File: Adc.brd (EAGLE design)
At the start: 96.8 x 28.7 mm, 98 parts, among them IC1 ADS1256IDBT, IC10 AD8605ARTZ, IC11 REF3125AIDBZT, IC12 MCP170333MB, IC2 ADUM1402ARWZ, IC3 AD8605ARTZ, IC4 AD8605ARTZ, IC5 AD8605ARTZ, IC6 AD8605ARTZ, IC7 AD8605ARTZ, IC8 AD8605ARTZ, IC9 AD8605ARTZ, Q1 7.68MHz

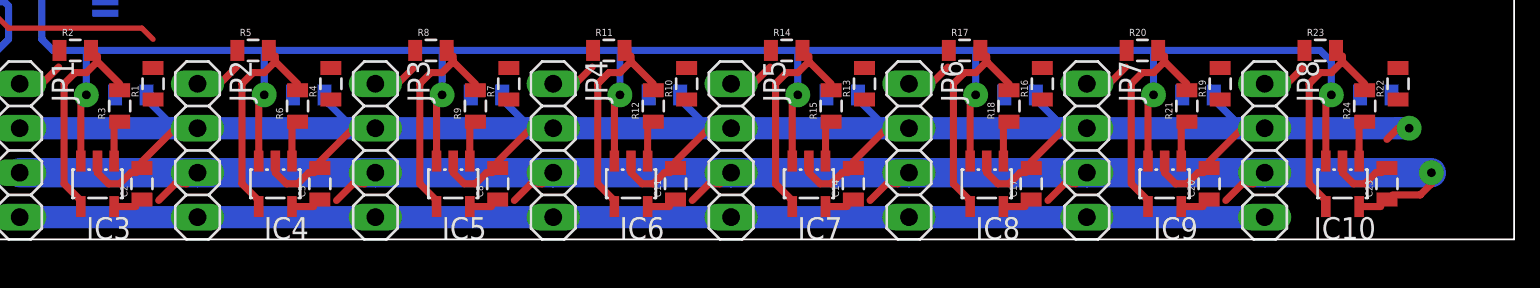
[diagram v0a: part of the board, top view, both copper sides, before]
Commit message: .
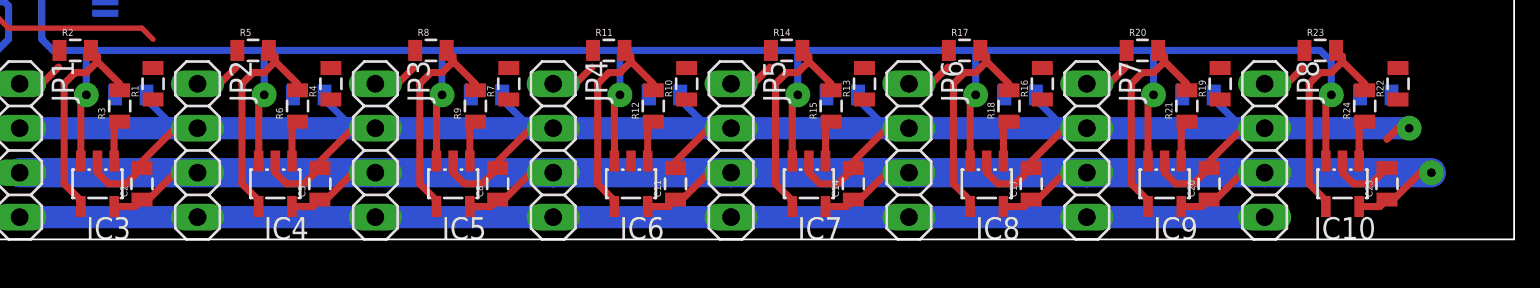
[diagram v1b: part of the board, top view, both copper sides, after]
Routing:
- net +5VA: track 139.3 -> 150.0 mm
